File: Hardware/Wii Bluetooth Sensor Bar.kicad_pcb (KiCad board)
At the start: 2 copper layers, 32 x 35.5 mm, 11 parts, among them U1 J27H002, U2 LM1117-3.3

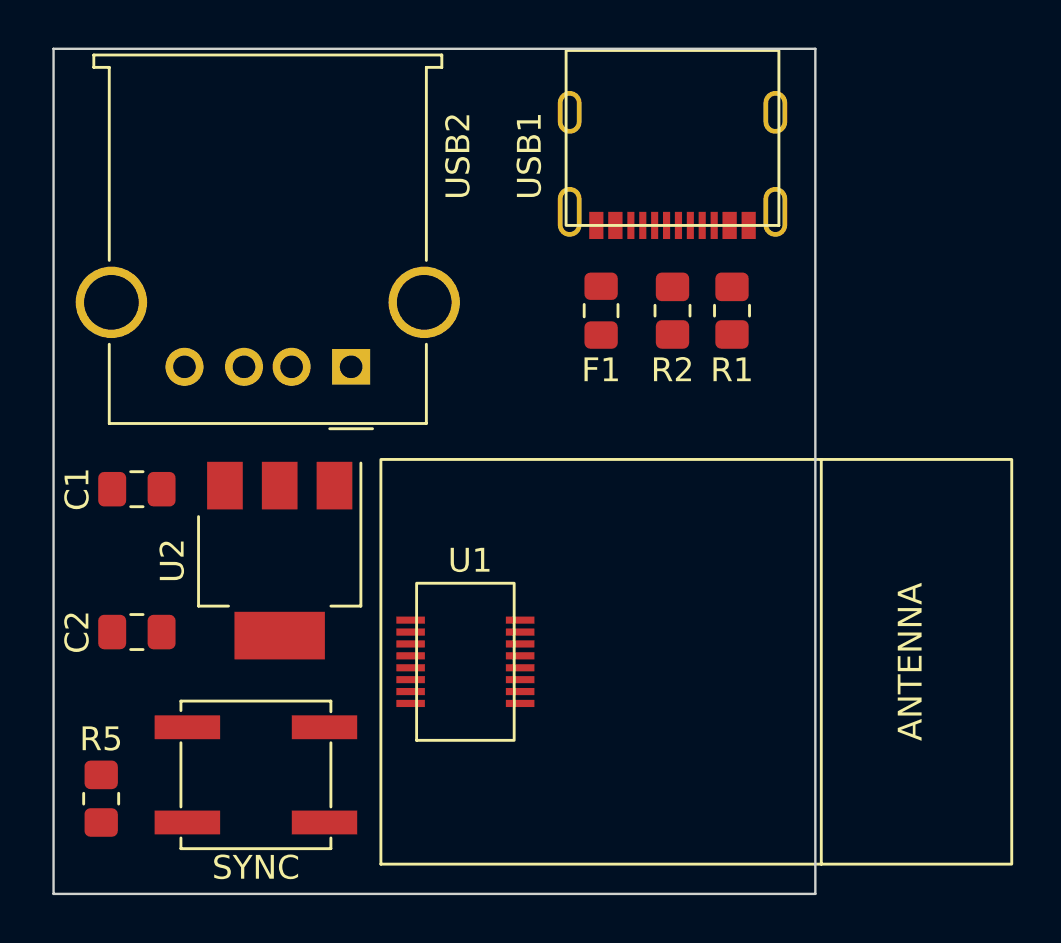
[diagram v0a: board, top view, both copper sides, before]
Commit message: Finish Rev A PCB
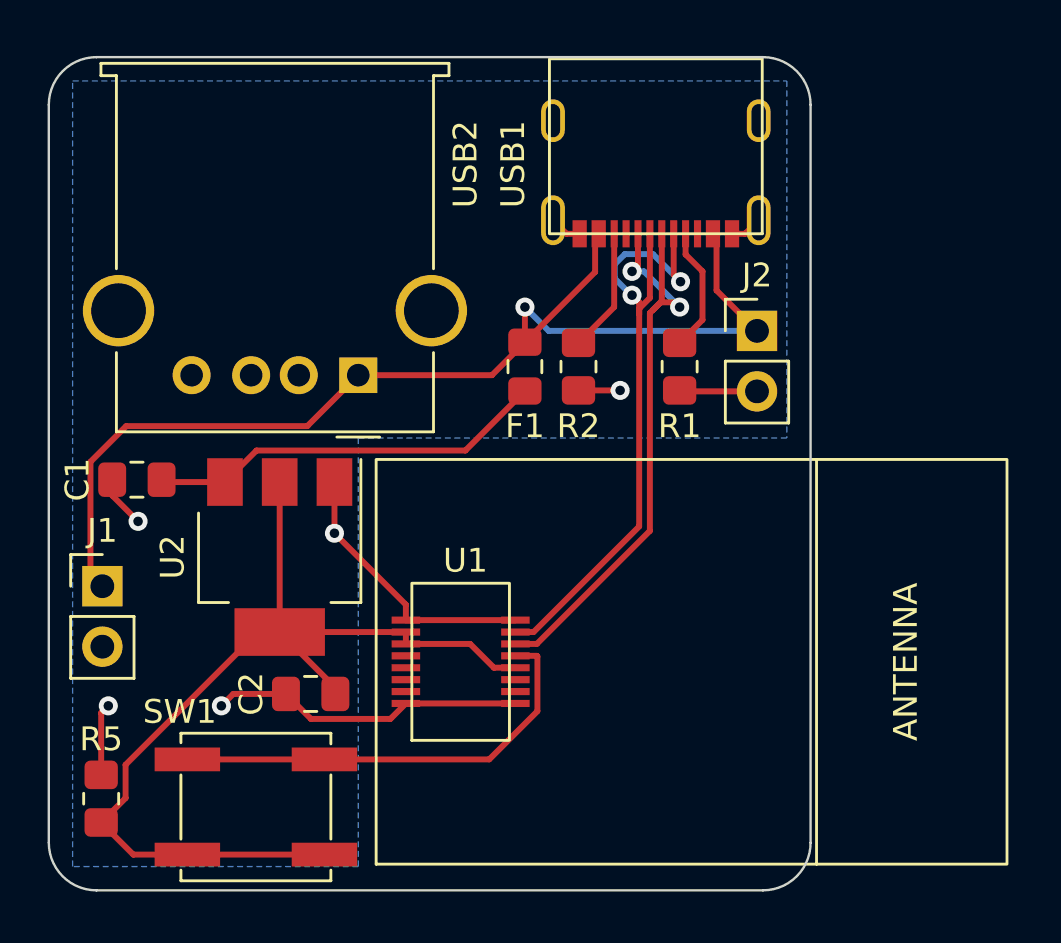
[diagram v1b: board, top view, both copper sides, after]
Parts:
- added J1: LED_Left, Connector_PinHeader_2.54mm:PinHeader_1x02_P2.54mm_Vertical, F.Cu at (125.2, 98.2)
- added J2: LED_Right, Connector_PinHeader_2.54mm:PinHeader_1x02_P2.54mm_Vertical, F.Cu at (152.8, 87.5)
- moved C2 7.75 mm to (134.0, 102.8)
- moved R2 4.60 mm to (145.2, 89.0)
- moved F1 3.97 mm to (143.0, 89.0)
- moved R1 3.22 mm to (149.5, 89.0)
- moved SW1 1.35 mm to (131.7, 107.5)
- moved USB1 0.78 mm to (152.8, 78.7)
- moved USB2 0.46 mm to (136.0, 89.4)
- moved C1 0.40 mm to (126.7, 93.8)
- moved U1 0.20 mm to (138.0, 103.2)
- moved U2 0.15 mm to (132.7, 97.0)
- renumbered SYNC to SW1
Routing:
- net +5V: track 0.00 -> 48.0 mm, vias 0 -> 1
- net +3V3: track 0.00 -> 42.3 mm
- net GND: track 0.00 -> 37.6 mm, vias 0 -> 5
- net Net-(USB1-PadA7): track 0.00 -> 27.6 mm, vias 0 -> 2
- net Net-(USB1-PadA6): track 0.00 -> 26.0 mm, vias 0 -> 2
- net Net-(SW1-Pad2): track 0.00 -> 18.8 mm
- net Net-(C1-Pad1): track 0.00 -> 16.9 mm
- net Net-(USB1-PadA5): track 0.00 -> 5.27 mm
- net Net-(USB1-PadB5): track 0.00 -> 5.20 mm
- added copper zone on B.Cu, net GND
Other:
- board size 32 x 35.5 mm -> 32 x 35 mm
